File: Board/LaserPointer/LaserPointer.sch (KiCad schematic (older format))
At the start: 17 parts, among them J1 S1, J2 S2, J3 S3, J4 Barrel_Jack, J5 LCD, U1 74HC595

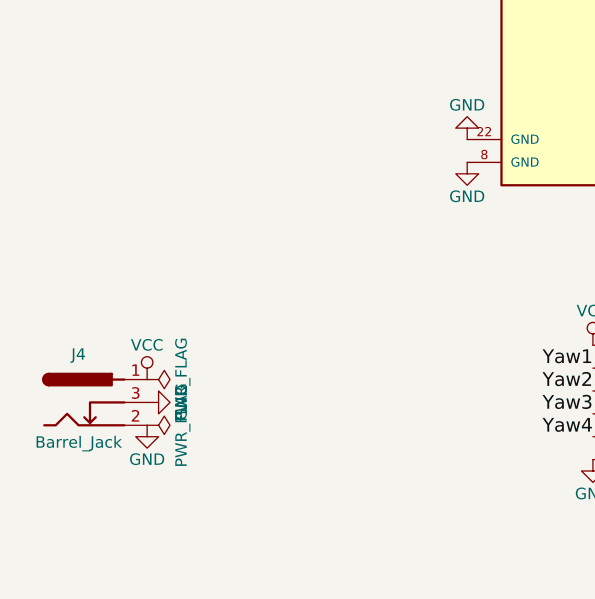
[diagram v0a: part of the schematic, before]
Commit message: Board updates
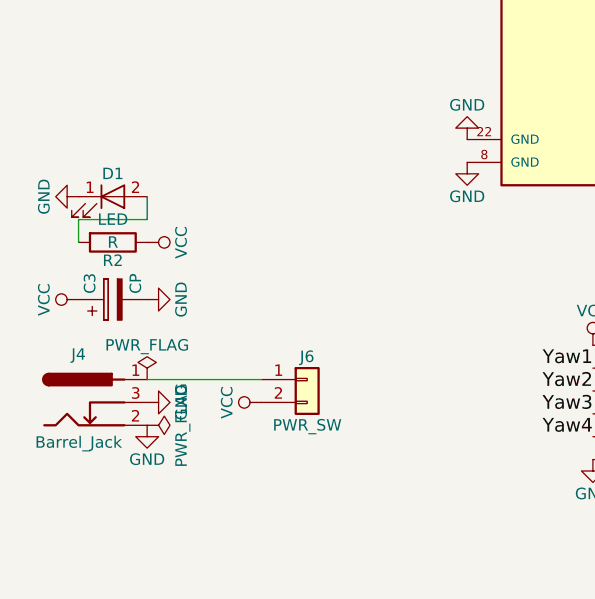
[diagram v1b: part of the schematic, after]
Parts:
- added C3: CP, Capacitors_THT:CP_Radial_D5.0mm_P2.00mm, symbol CP
- added D1: LED, LEDs:LED_0603_HandSoldering, symbol LED
- added J6: PWR_SW, Pin_Headers:Pin_Header_Straight_1x02_Pitch2.54mm, symbol Conn_01x02
- added R2: R, Resistors_SMD:R_0603_HandSoldering, symbol R
- C1, C2: footprint Capacitors_THT:C_Disc_D6.0mm_W2.5mm_P5.00mm -> Capacitors_SMD:C_0603_HandSoldering
- R1: footprint Resistors_THT:R_Axial_DIN0207_L6.3mm_D2.5mm_P7.62mm_Horizontal -> Resistors_SMD:R_0603_HandSoldering
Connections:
- net GND: now also C3.2, D1.1 (K)
- net VCC: now also C3.1, J6.2 (Pin_2), R2.1; no longer J4.1
- new net: J4.1, J6.1 (Pin_1)
- new net: D1.2 (A), R2.2
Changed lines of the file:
@@
 EELAYER 25 0
 EELAYER END
-$Descr A4 11693 8268
+$Descr USLetter 11000 8500
 encoding utf-8
 Sheet 1 1
 Title ""
 Date ""
-Rev ""
+Rev "1"
 Comp ""
 Comment1 ""
@@
 F 0 "C1" H 6060 1920 50  0000 L CNN
 F 1 "22pF" H 6060 1770 50  0000 L CNN
-F 2 "Capacitors_THT:C_Disc_D6.0mm_W2.5mm_P5.00mm" H 6050 1850 50  0001 C CNN
+F 2 "Capacitors_SMD:C_0603_HandSoldering" H 6050 1850 50  0001 C CNN
 F 3 "" H 6050 1850 50  0001 C CNN
 	1    6050 1850
@@
 F 0 "C2" H 6060 2120 50  0000 L CNN
 F 1 "22pF" H 6060 1970 50  0000 L CNN
-F 2 "Capacitors_THT:C_Disc_D6.0mm_W2.5mm_P5.00mm" H 6050 2050 50  0001 C CNN
+F 2 "Capacitors_SMD:C_0603_HandSoldering" H 6050 2050 50  0001 C CNN
 F 3 "" H 6050 2050 50  0001 C CNN
 	1    6050 2050
@@
 SPI_SCK
 $Comp
-L VCC #PWR021
-U 1 1 5A8C90D4
-P 1100 4550
-F 0 "#PWR021" H 1100 4400 50  0001 C CNN
-F 1 "VCC" H 1100 4700 50  0000 C CNN
-F 2 "" H 1100 4550 50  0001 C CNN
-F 3 "" H 1100 4550 50  0001 C CNN
-	1    1100 4550
-	1    0    0    -1
-$EndComp
-$Comp
-L GND #PWR022
+L GND #PWR021
 U 1 1 5A8C910F
 P 1100 4750
-F 0 "#PWR022" H 1100 4500 50  0001 C CNN
+F 0 "#PWR021" H 1100 4500 50  0001 C CNN
 F 1 "GND" H 1100 4600 50  0000 C CNN
 F 2 "" H 1100 4750 50  0001 C CNN
@@
 $EndComp
 $Comp
-L PWR_FLAG #FLG023
-U 1 1 5A8C914A
-P 1100 4550
-F 0 "#FLG023" H 1100 4625 50  0001 C CNN
-F 1 "PWR_FLAG" H 1100 4700 50  0000 C CNN
-F 2 "" H 1100 4550 50  0001 C CNN
-F 3 "" H 1100 4550 50  0001 C CNN
-	1    1100 4550
-	0    1    1    0
-$EndComp
-$Comp
-L PWR_FLAG #FLG024
+L PWR_FLAG #FLG022
 U 1 1 5A8C9185
 P 1100 4750
-F 0 "#FLG024" H 1100 4825 50  0001 C CNN
+F 0 "#FLG022" H 1100 4825 50  0001 C CNN
 F 1 "PWR_FLAG" H 1100 4900 50  0000 C CNN
 F 2 "" H 1100 4750 50  0001 C CNN
@@
 	5300 2100 5950 2100
 $Comp
-L GND #PWR025
+L GND #PWR023
 U 1 1 5A8C942B
 P 6150 2050
-F 0 "#PWR025" H 6150 1800 50  0001 C CNN
+F 0 "#PWR023" H 6150 1800 50  0001 C CNN
 F 1 "GND" H 6150 1900 50  0000 C CNN
 F 2 "" H 6150 2050 50  0001 C CNN
@@
 $EndComp
 $Comp
-L GND #PWR026
+L GND #PWR024
 U 1 1 5A8C9466
 P 6150 1850
-F 0 "#PWR026" H 6150 1600 50  0001 C CNN
+F 0 "#PWR024" H 6150 1600 50  0001 C CNN
 F 1 "GND" H 6150 1700 50  0000 C CNN
 F 2 "" H 6150 1850 50  0001 C CNN
@@
 F 0 "R1" V 4630 2750 50  0000 C CNN
 F 1 "10k" V 4550 2750 50  0000 C CNN
-F 2 "Resistors_THT:R_Axial_DIN0207_L6.3mm_D2.5mm_P7.62mm_Horizontal" V 4480 2750 50  0001 C CNN
+F 2 "Resistors_SMD:R_0603_HandSoldering" V 4480 2750 50  0001 C CNN
 F 3 "" H 4550 2750 50  0001 C CNN
 	1    4550 2750
@@
 $EndComp
 $Comp
-L VCC #PWR027
+L VCC #PWR025
 U 1 1 5A8C9656
 P 4700 2750
-F 0 "#PWR027" H 4700 2600 50  0001 C CNN
+F 0 "#PWR025" H 4700 2600 50  0001 C CNN
 F 1 "VCC" H 4700 2900 50  0000 C CNN
 F 2 "" H 4700 2750 50  0001 C CNN
@@
 $EndComp
 $Comp
-L GND #PWR028
+L GND #PWR026
 U 1 1 5A8C97A9
 P 5600 2650
-F 0 "#PWR028" H 5600 2400 50  0001 C CNN
+F 0 "#PWR026" H 5600 2400 50  0001 C CNN
 F 1 "GND" H 5600 2500 50  0000 C CNN
 F 2 "" H 5600 2650 50  0001 C CNN
@@
 $EndComp
 $Comp
-L GND #PWR029
+L GND #PWR027
 U 1 1 5A8C97F0
 P 6150 2550
-F 0 "#PWR029" H 6150 2300 50  0001 C CNN
+F 0 "#PWR027" H 6150 2300 50  0001 C CNN
 F 1 "GND" H 6150 2400 50  0000 C CNN
 F 2 "" H 6150 2550 50  0001 C CNN
@@
 $EndComp
 $Comp
-L GND #PWR030
+L GND #PWR028
 U 1 1 5A8C9837
 P 6700 2450
-F 0 "#PWR030" H 6700 2200 50  0001 C CNN
+F 0 "#PWR028" H 6700 2200 50  0001 C CNN
 F 1 "GND" H 6700 2300 50  0000 C CNN
 F 2 "" H 6700 2450 50  0001 C CNN
@@
 	4400 2350 6700 2350
 $Comp
-L VCC #PWR031
+L VCC #PWR029
 U 1 1 5A8CBD31
 P 2500 1600
-F 0 "#PWR031" H 2500 1450 50  0001 C CNN
+F 0 "#PWR029" H 2500 1450 50  0001 C CNN
 F 1 "VCC" H 2500 1750 50  0000 C CNN
 F 2 "" H 2500 1600 50  0001 C CNN
@@
 $EndComp
 $Comp
-L VCC #PWR032
+L VCC #PWR030
 U 1 1 5A8CBD78
 P 2500 1900
-F 0 "#PWR032" H 2500 1750 50  0001 C CNN
+F 0 "#PWR030" H 2500 1750 50  0001 C CNN
 F 1 "VCC" H 2500 2050 50  0000 C CNN
 F 2 "" H 2500 1900 50  0001 C CNN
@@
 $EndComp
 $Comp
-L GND #PWR033
+L GND #PWR031
 U 1 1 5A8CBDBF
 P 1100 4650
-F 0 "#PWR033" H 1100 4400 50  0001 C CNN
+F 0 "#PWR031" H 1100 4400 50  0001 C CNN
 F 1 "GND" H 1100 4500 50  0000 C CNN
 F 2 "" H 1100 4650 50  0001 C CNN
@@
 $EndComp
 $Comp
-L GND #PWR034
+L GND #PWR032
 U 1 1 5A8CBE7D
 P 2500 3500
-F 0 "#PWR034" H 2500 3250 50  0001 C CNN
+F 0 "#PWR032" H 2500 3250 50  0001 C CNN
 F 1 "GND" H 2500 3350 50  0000 C CNN
 F 2 "" H 2500 3500 50  0001 C CNN
@@
 	-1   0    0    1
 $EndComp
+$Comp
+L LED D1
+U 1 1 5A8C73D3
+P 950 3750
+F 0 "D1" H 950 3850 50  0000 C CNN
+F 1 "LED" H 950 3650 50  0000 C CNN
+F 2 "LEDs:LED_0603_HandSoldering" H 950 3750 50  0001 C CNN
+F 3 "" H 950 3750 50  0001 C CNN
+	1    950  3750
+	1    0    0    -1
+$EndComp
+$Comp
+L CP C3
+U 1 1 5A8C743C
+P 950 4200
+F 0 "C3" H 975 4300 50  0000 L CNN
+F 1 "CP" H 975 4100 50  0000 L CNN
+F 2 "Capacitors_THT:CP_Radial_D5.0mm_P2.00mm" H 988 4050 50  0001 C CNN
+F 3 "" H 950 4200 50  0001 C CNN
+	1    950  4200
+	0    -1   -1   0
+$EndComp
+$Comp
+L R R2
+U 1 1 5A8C74C1
+P 950 3950
+F 0 "R2" V 1030 3950 50  0000 C CNN
+F 1 "R" V 950 3950 50  0000 C CNN
+F 2 "Resistors_SMD:R_0603_HandSoldering" V 880 3950 50  0001 C CNN
+F 3 "" H 950 3950 50  0001 C CNN
+	1    950  3950
+	0    1    1    0
+$EndComp
+Wire Wire Line
+	800  3950 800  3850
+Wire Wire Line
+	800  3850 1100 3850
+Wire Wire Line
+	1100 3850 1100 3750
+$Comp
+L GND #PWR033
+U 1 1 5A8C794F
+P 1100 4200
+F 0 "#PWR033" H 1100 3950 50  0001 C CNN
+F 1 "GND" H 1100 4050 50  0000 C CNN
+F 2 "" H 1100 4200 50  0001 C CNN
+F 3 "" H 1100 4200 50  0001 C CNN
+	1    1100 4200
+	0    -1   -1   0
+$EndComp
+$Comp
+L GND #PWR034
+U 1 1 5A8C799F
+P 800 3750
+F 0 "#PWR034" H 800 3500 50  0001 C CNN
+F 1 "GND" H 800 3600 50  0000 C CNN
+F 2 "" H 800 3750 50  0001 C CNN
+F 3 "" H 800 3750 50  0001 C CNN
+	1    800  3750
+	0    1    1    0
+$EndComp
+$Comp
+L VCC #PWR035
+U 1 1 5A8C7AA7
+P 800 4200
+F 0 "#PWR035" H 800 4050 50  0001 C CNN
+F 1 "VCC" H 800 4350 50  0000 C CNN
+F 2 "" H 800 4200 50  0001 C CNN
+F 3 "" H 800 4200 50  0001 C CNN
+	1    800  4200
+	0    -1   -1   0
+$EndComp
+$Comp
+L VCC #PWR036
+U 1 1 5A8C7AF7
+P 1100 3950
+F 0 "#PWR036" H 1100 3800 50  0001 C CNN
+F 1 "VCC" H 1100 4100 50  0000 C CNN
+F 2 "" H 1100 3950 50  0001 C CNN
+F 3 "" H 1100 3950 50  0001 C CNN
+	1    1100 3950
+	0    1    1    0
+$EndComp
+$Comp
+L Conn_01x02 J6
+U 1 1 5A8C7D54
+P 1800 4550
+F 0 "J6" H 1800 4650 50  0000 C CNN
+F 1 "PWR_SW" H 1800 4350 50  0000 C CNN
+F 2 "Pin_Headers:Pin_Header_Straight_1x02_Pitch2.54mm" H 1800 4550 50  0001 C CNN
+F 3 "" H 1800 4550 50  0001 C CNN
+	1    1800 4550
+	1    0    0    -1
+$EndComp
+Wire Wire Line
+	1100 4550 1600 4550
+$Comp
+L VCC #PWR037
+U 1 1 5A8C7E1A
+P 1600 4650
+F 0 "#PWR037" H 1600 4500 50  0001 C CNN
+F 1 "VCC" H 1600 4800 50  0000 C CNN
+F 2 "" H 1600 4650 50  0001 C CNN
+F 3 "" H 1600 4650 50  0001 C CNN
+	1    1600 4650
+	0    -1   -1   0
+$EndComp
+$Comp
+L PWR_FLAG #FLG038
+U 1 1 5A8C7E6D
+P 1100 4550
+F 0 "#FLG038" H 1100 4625 50  0001 C CNN
+F 1 "PWR_FLAG" H 1100 4700 50  0000 C CNN
+F 2 "" H 1100 4550 50  0001 C CNN
+F 3 "" H 1100 4550 50  0001 C CNN
+	1    1100 4550
+	1    0    0    -1
+$EndComp
 $EndSCHEMATC
